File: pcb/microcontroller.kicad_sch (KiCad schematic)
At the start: 22 parts, among them U2 STM32G431CBTx, U3 USBLC6-2SC6, Y1 24Mhz

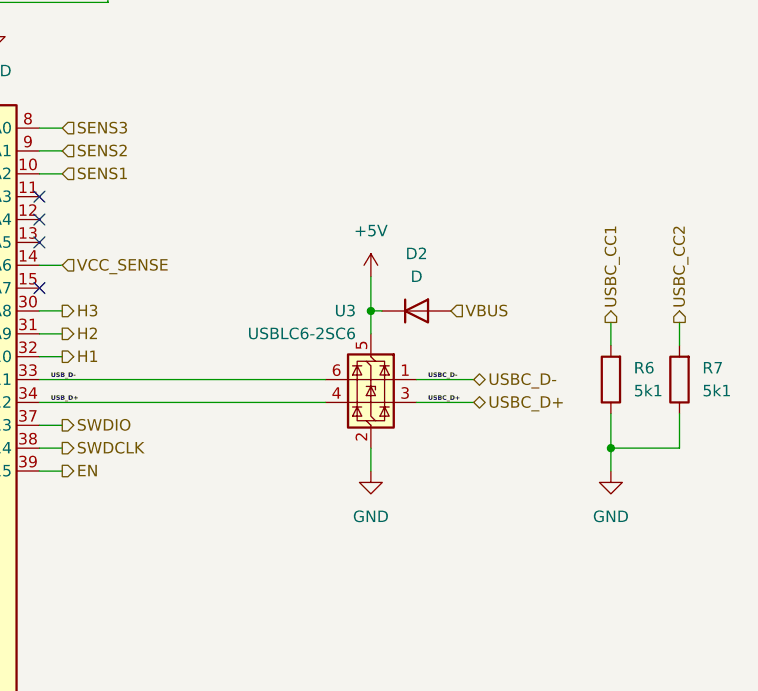
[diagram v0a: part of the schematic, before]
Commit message: pcb: v1.0 layout finsihed
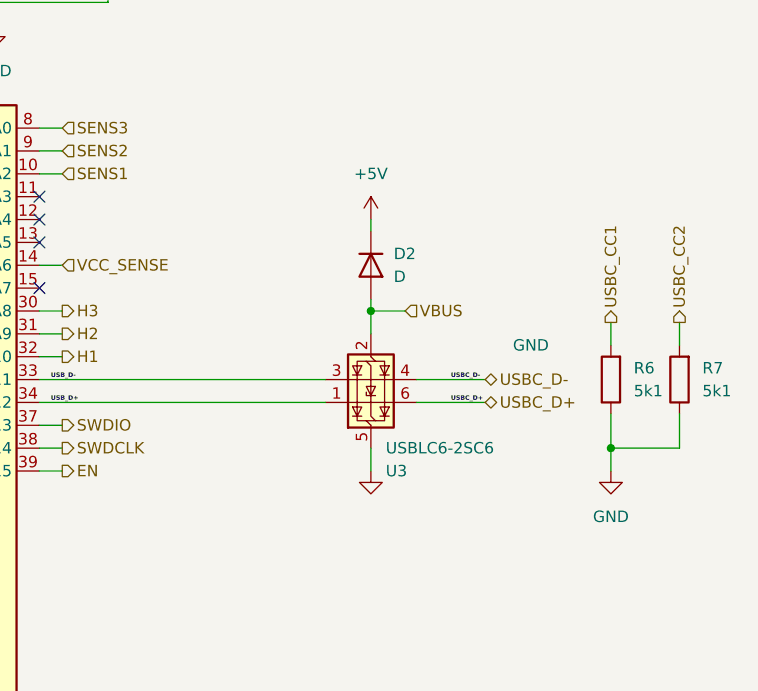
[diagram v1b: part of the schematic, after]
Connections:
- net +5V: no longer U3.5 (VBUS)
- net GND: now also U3.5 (VBUS); no longer U3.2 (GND)
- net USBC_D+: now also U3.6 (I/O1); no longer U3.3 (I/O2)
- net USBC_D-: now also U3.4 (I/O2); no longer U3.1 (I/O1)
- net USB_D+: now also U3.1 (I/O1); no longer U3.4 (I/O2)
- net USB_D-: now also U3.3 (I/O2); no longer U3.6 (I/O1)
- net VBUS: now also U3.2 (GND)
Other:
- moved on the sheet: D2
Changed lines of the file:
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@@
 	)
 	(junction
-		(at 68.58 104.14)
+		(at 193.04 93.98)
 		(diameter 0)
 		(color 0 0 0 0)
 	)
 	(junction
-		(at 120.65 73.66)
+		(at 68.58 104.14)
 		(diameter 0)
 		(color 0 0 0 0)
 	)
 	(junction
-		(at 138.43 66.04)
+		(at 120.65 73.66)
 		(diameter 0)
 		(color 0 0 0 0)
 	)
 	(junction
-		(at 193.04 93.98)
+		(at 138.43 66.04)
 		(diameter 0)
 		(color 0 0 0 0)
@@
 	(wire
 		(pts
-			(xy 193.04 93.98) (xy 194.31 93.98)
-		)
-		(stroke
-			(width 0)
-			(type default)
-		)
-	)
-	(wire
-		(pts
 			(xy 120.65 137.16) (xy 123.19 137.16)
 		)
@@
 	(wire
 		(pts
-			(xy 193.04 109.22) (xy 193.04 111.76)
+			(xy 198.12 101.6) (xy 205.74 101.6)
 		)
 		(stroke
@@
 	(wire
 		(pts
-			(xy 193.04 90.17) (xy 193.04 93.98)
+			(xy 193.04 109.22) (xy 193.04 111.76)
 		)
 		(stroke
@@
 	(wire
 		(pts
-			(xy 120.65 91.44) (xy 123.19 91.44)
+			(xy 193.04 83.82) (xy 193.04 85.09)
 		)
 		(stroke
@@
 	(wire
 		(pts
-			(xy 140.97 147.32) (xy 140.97 149.86)
+			(xy 120.65 91.44) (xy 123.19 91.44)
 		)
 		(stroke
@@
 	(wire
 		(pts
-			(xy 86.36 119.38) (xy 99.06 119.38)
+			(xy 140.97 147.32) (xy 140.97 149.86)
 		)
 		(stroke
@@
 	(wire
 		(pts
-			(xy 198.12 101.6) (xy 204.47 101.6)
+			(xy 86.36 119.38) (xy 99.06 119.38)
 		)
 		(stroke
@@
 	(wire
 		(pts
-			(xy 193.04 96.52) (xy 193.04 93.98)
-		)
-		(stroke
-			(width 0)
-			(type default)
-		)
-	)
-	(wire
-		(pts
 			(xy 80.01 114.3) (xy 80.01 123.19)
 		)
@@
 	(wire
 		(pts
+			(xy 193.04 93.98) (xy 193.04 96.52)
+		)
+		(stroke
+			(width 0)
+			(type default)
+		)
+	)
+	(wire
+		(pts
+			(xy 193.04 93.98) (xy 196.85 93.98)
+		)
+		(stroke
+			(width 0)
+			(type default)
+		)
+	)
+	(wire
+		(pts
 			(xy 100.33 46.99) (xy 113.03 46.99)
 		)
@@
 	(wire
 		(pts
+			(xy 198.12 104.14) (xy 205.74 104.14)
+		)
+		(stroke
+			(width 0)
+			(type default)
+		)
+	)
+	(wire
+		(pts
 			(xy 100.33 49.53) (xy 100.33 46.99)
 		)
@@
 	(wire
 		(pts
+			(xy 193.04 92.71) (xy 193.04 93.98)
+		)
+		(stroke
+			(width 0)
+			(type default)
+		)
+	)
+	(wire
+		(pts
 			(xy 77.47 116.84) (xy 88.9 116.84)
 		)
@@
 	(wire
 		(pts
-			(xy 198.12 104.14) (xy 204.47 104.14)
-		)
-		(stroke
-			(width 0)
-			(type default)
-		)
-	)
-	(wire
-		(pts
 			(xy 219.71 109.22) (xy 227.33 109.22)
 		)
@@
 	)
 	(label "USBC_D+"
-		(at 199.39 104.14 0)
+		(at 201.93 104.14 0)
 		(fields_autoplaced yes)
 		(effects
@@
 	)
 	(label "USBC_D-"
-		(at 199.39 101.6 0)
+		(at 201.93 101.6 0)
 		(fields_autoplaced yes)
 		(effects
@@
 	(hierarchical_label "USBC_D+"
 		(shape bidirectional)
-		(at 204.47 104.14 0)
+		(at 205.74 104.14 0)
 		(fields_autoplaced yes)
 		(effects
@@
 	(hierarchical_label "USBC_D-"
 		(shape bidirectional)
-		(at 204.47 101.6 0)
+		(at 205.74 101.6 0)
 		(fields_autoplaced yes)
 		(effects
@@
 	(hierarchical_label "VBUS"
 		(shape input)
-		(at 201.93 93.98 0)
+		(at 196.85 93.98 0)
 		(fields_autoplaced yes)
 		(effects
@@
 	(symbol
 		(lib_id "Power_Protection:USBLC6-2SC6")
-		(at 193.04 101.6 0)
-		(mirror y)
+		(at 193.04 104.14 0)
+		(mirror x)
 		(unit 1)
 		(exclude_from_sim no)
@@
 		(fields_autoplaced yes)
 		(property "Reference" "U3"
-			(at 191.3889 93.98 0)
+			(at 194.6911 111.76 0)
 			(effects
 				(font
@@
 		)
 		(property "Value" "USBLC6-2SC6"
-			(at 191.3889 96.52 0)
+			(at 194.6911 109.22 0)
 			(effects
 				(font
@@
 		)
 		(property "Footprint" "Package_TO_SOT_SMD:SOT-23-6"
-			(at 191.77 107.95 0)
+			(at 194.31 97.79 0)
 			(effects
 				(font
@@
 		)
 		(property "Datasheet" "https://www.st.com/resource/en/datasheet/usblc6-2.pdf"
-			(at 191.77 109.855 0)
+			(at 194.31 95.885 0)
 			(effects
 				(font
@@
 		)
 		(property "Description" "Very low capacitance ESD protection diode, 2 data-line, SOT-23-6"
-			(at 193.04 101.6 0)
+			(at 193.04 104.14 0)
 			(effects
 				(font
@@
 	(symbol
 		(lib_id "power:+5V")
-		(at 193.04 90.17 0)
+		(at 193.04 83.82 0)
 		(unit 1)
 		(exclude_from_sim no)
@@
 		(fields_autoplaced yes)
 		(property "Reference" "#PWR020"
-			(at 193.04 93.98 0)
+			(at 193.04 87.63 0)
 			(effects
 				(font
@@
 		)
 		(property "Value" "+5V"
-			(at 193.04 85.09 0)
+			(at 193.04 78.74 0)
 			(effects
 				(font
@@
 		)
 		(property "Footprint" ""
-			(at 193.04 90.17 0)
+			(at 193.04 83.82 0)
 			(effects
 				(font
@@
 		)
 		(property "Datasheet" ""
-			(at 193.04 90.17 0)
+			(at 193.04 83.82 0)
 			(effects
 				(font
@@
 		)
 		(property "Description" "Power symbol creates a global label with name \"+5V\""
-			(at 193.04 90.17 0)
+			(at 193.04 83.82 0)
 			(effects
 				(font
@@
 		(on_board yes)
 		(dnp no)
-		(fields_autoplaced yes)
 		(property "Reference" "#PWR018"
 			(at 193.04 118.11 0)
@@
 		)
 		(property "Value" "GND"
-			(at 193.04 116.84 0)
+			(at 210.82 97.79 0)
 			(effects
 				(font
@@
 	(symbol
 		(lib_id "Device:D")
-		(at 198.12 93.98 0)
+		(at 193.04 88.9 270)
 		(unit 1)
 		(exclude_from_sim no)
@@
 		(fields_autoplaced yes)
 		(property "Reference" "D2"
-			(at 198.12 87.63 0)
+			(at 195.58 87.6299 90)
 			(effects
 				(font
 					(size 1.27 1.27)
 				)
+				(justify left)
 			)
 		)
 		(property "Value" "D"
-			(at 198.12 90.17 0)
+			(at 195.58 90.1699 90)
 			(effects
 				(font
 					(size 1.27 1.27)
 				)
+				(justify left)
 			)
 		)
 		(property "Footprint" "Diode_SMD:D_MiniMELF"
-			(at 198.12 93.98 0)
+			(at 193.04 88.9 0)
 			(effects
 				(font
@@
 		)
 		(property "Datasheet" "~"
-			(at 198.12 93.98 0)
+			(at 193.04 88.9 0)
 			(effects
 				(font
@@
 		)
 		(property "Description" "Diode"
-			(at 198.12 93.98 0)
+			(at 193.04 88.9 0)
 			(effects
 				(font
@@
 		)
 		(property "Sim.Device" "D"
-			(at 198.12 93.98 0)
+			(at 193.04 88.9 0)
 			(effects
 				(font
@@
 		)
 		(property "Sim.Pins" "1=K 2=A"
-			(at 198.12 93.98 0)
+			(at 193.04 88.9 0)
 			(effects
 				(font
